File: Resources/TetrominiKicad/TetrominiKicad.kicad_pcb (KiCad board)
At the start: 2 copper layers, 99.5 x 86 mm, 45 parts, among them SW1 POWER_PUSH_SPDT

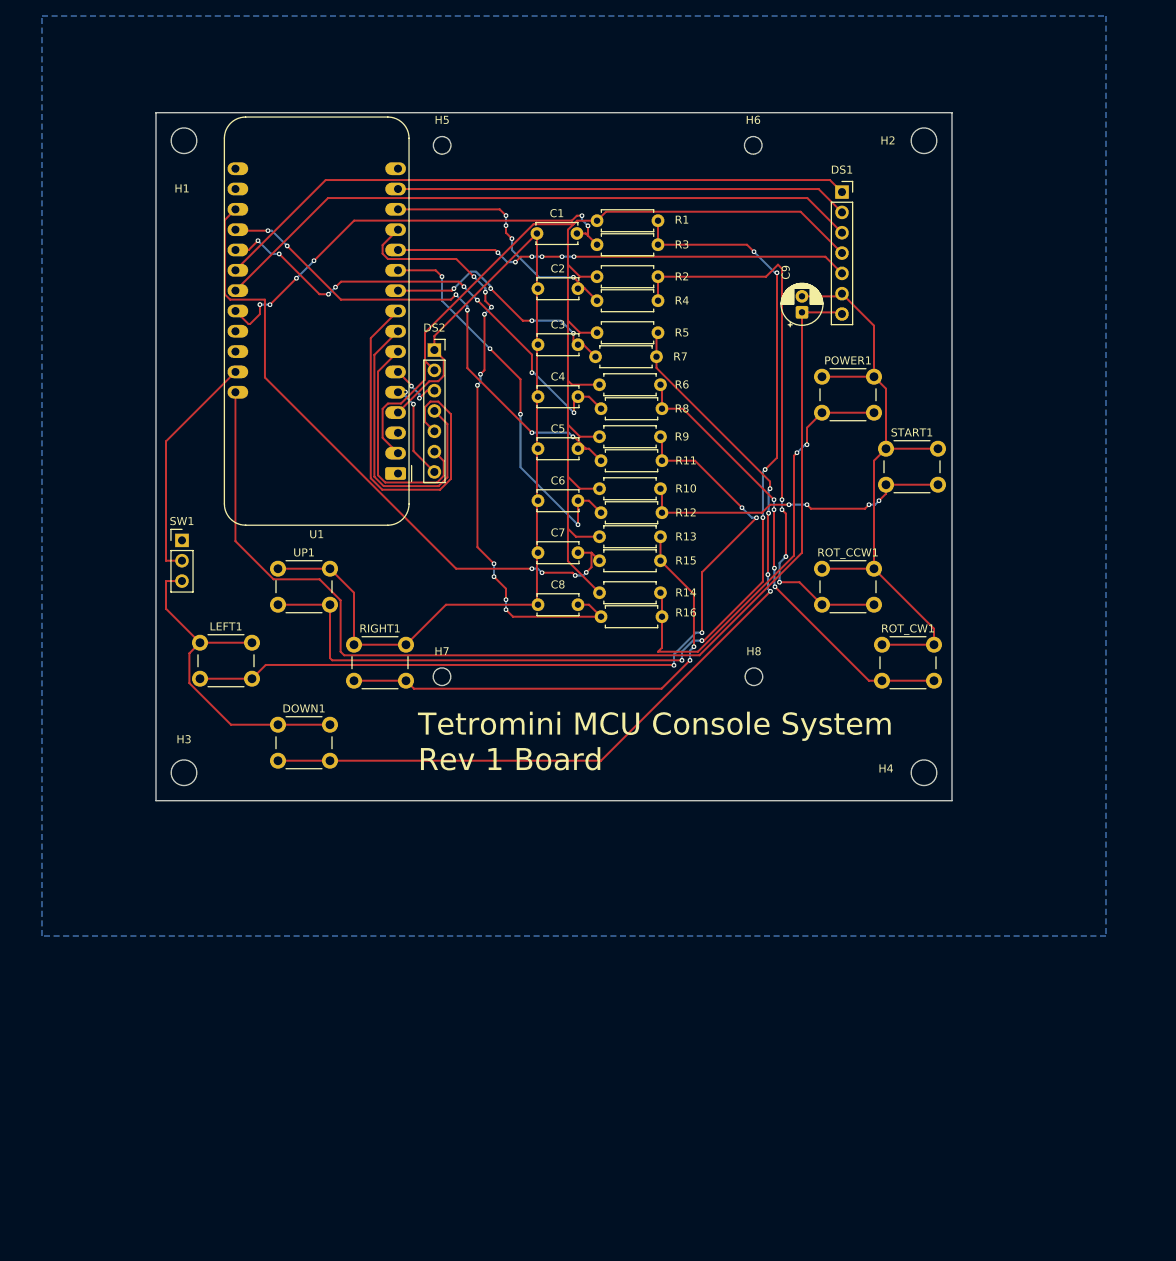
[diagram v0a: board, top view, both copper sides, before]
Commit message: Rev 1a PCB Update
PCB is now Tetromino-shaped!!!!! Also was sent to OSH Park, it's awaiting printing. Excited!!!! Added actual part numbers to BoM as well.
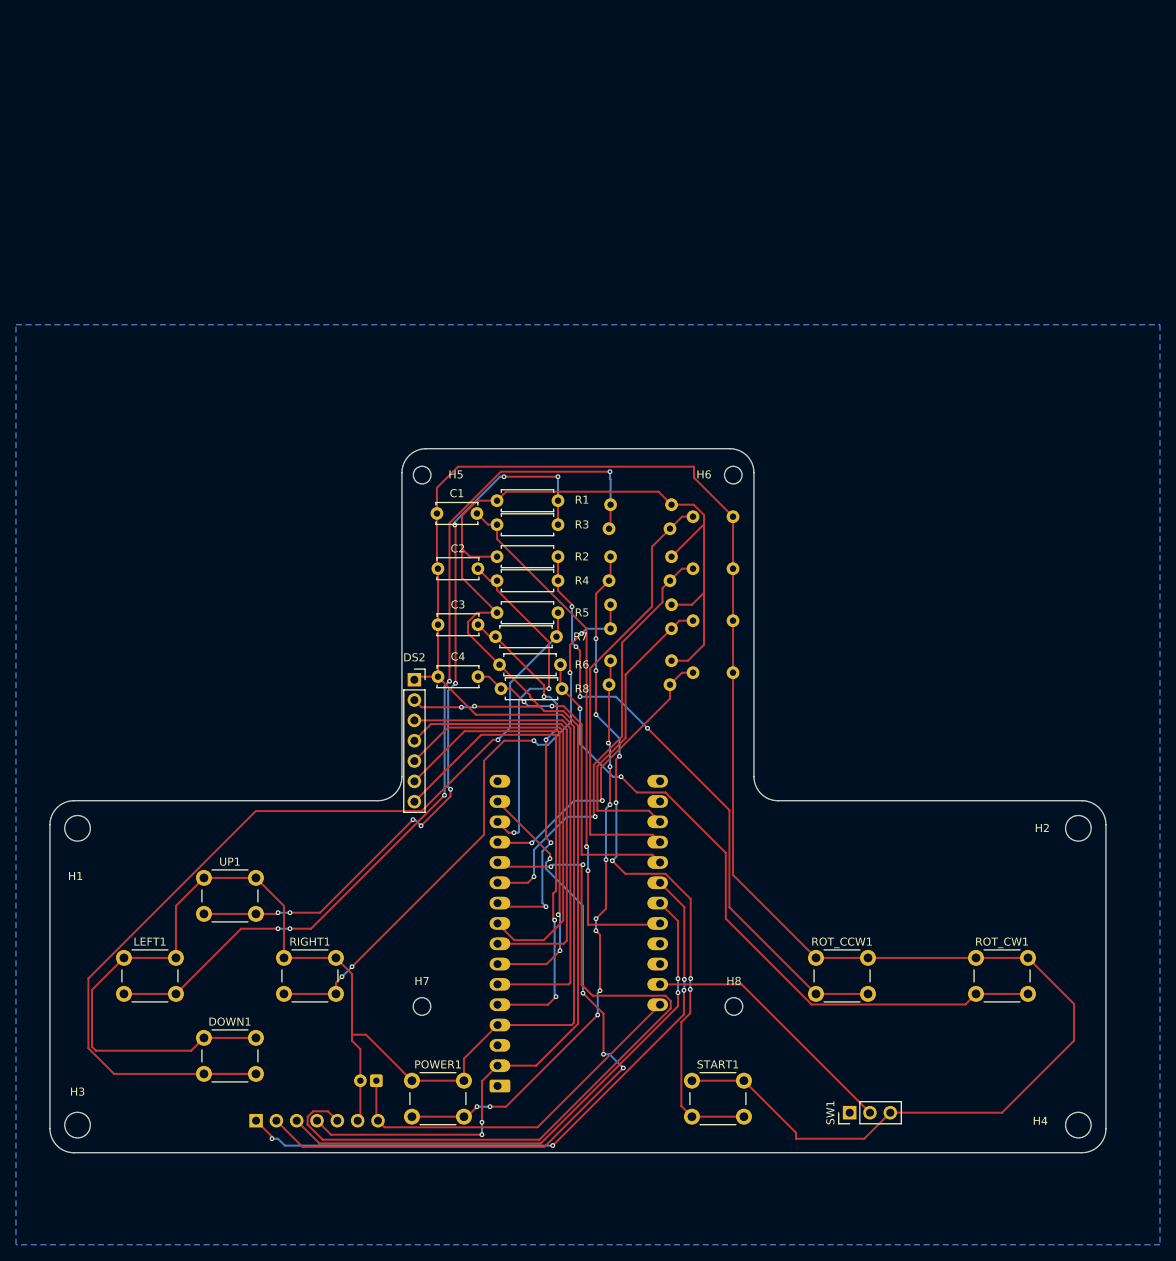
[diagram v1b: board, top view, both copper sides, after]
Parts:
- C5, C6, C7, C8, C9, DS1, R10, R11, R12, R13, R14, R15, R16, R9, U1: moved to B.Cu
- moved DS1 137.3 mm to (43.3, 165.0), turned to -90 degrees
- moved SW1 109.9 mm to (117.5, 164.0), turned to 90 degrees
- moved C9 109.8 mm to (58.3, 160.0), turned to 180 degrees
- moved POWER1 101.8 mm to (62.8, 160.0)
- moved H2 88.1 mm to (146.1, 128.5)
- moved H1 87.0 mm to (21.0, 128.5)
- moved START1 82.6 mm to (97.8, 160.0)
- moved U1 77.6 mm to (73.5, 160.7), turned to 0 degrees
- moved ROT_CCW1 48.7 mm to (113.3, 144.7)
- moved H4 48.1 mm to (146.1, 165.6)
- moved H3 46.0 mm to (21.0, 165.6)
- moved H5 41.3 mm to (64.0, 84.3)
- moved H6 41.3 mm to (102.9, 84.3)
- moved DS2 41.3 mm to (63.1, 109.9)
- moved H7 41.3 mm to (64.0, 150.7)
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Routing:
- net GND: track 244.3 -> 412.8 mm
- net AUDIO_VIN: track 139.6 -> 47.0 mm
- net SPI_SCK: track 6.65 -> 60.9 mm, vias 2 -> 0
- net ~{OLED_CHIP_SELECT}: track 12.4 -> 61.9 mm
- net +3.3V: track 155.4 -> 203.8 mm, vias 0 -> 4
- net Net-(R10-Pad2): track 40.1 -> 86.9 mm, vias 4 -> 8
- net BTN_RIGHT: track 82.6 -> 38.1 mm, vias 4 -> 0
- net ~{AUDIO_SHUTDOWN}: track 57.3 -> 97.4 mm, vias 6 -> 2
- net BTN_POWER: track 76.9 -> 37.0 mm, vias 10 -> 2
- net Net-(R1-Pad2): track 130.8 -> 93.6 mm, vias 6 -> 9
- net AUDIO_BITCLK: track 56.7 -> 89.5 mm, vias 0 -> 4
- net Net-(R6-Pad2): track 57.5 -> 85.8 mm, vias 4 -> 2
- net OLED_DATA_CMD: track 29.0 -> 56.7 mm, vias 0 -> 2
- net Net-(POWER1-Pad2): track 55.6 -> 74.0 mm, vias 2 -> 10
- net ROT_CW: track 60.0 -> 41.9 mm, vias 8 -> 2
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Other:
- board size 99.5 x 86 mm -> 132 x 88 mm
- board text added: "Tetromini MCU Console System Rev 1a Board"
- board text removed: "Tetromini MCU Console System Rev 1 Board"
